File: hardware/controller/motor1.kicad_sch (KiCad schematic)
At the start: 55 parts, among them J5 Conn_01x01, J6 Conn_01x01, J7 Conn_01x01, J8 Conn_01x09, Q2 IPD90N04S4L04, Q3 IPD90N04S4L04, Q4 IPD90N04S4L04, Q5 IPD90N04S4L04, Q6 IPD90N04S4L04, Q7 IPD90N04S4L04, U10 MCP6541, U11 LM2105D, U12 MCP6541, U13 LM2105D, U8 MCP6541, U9 LM2105D

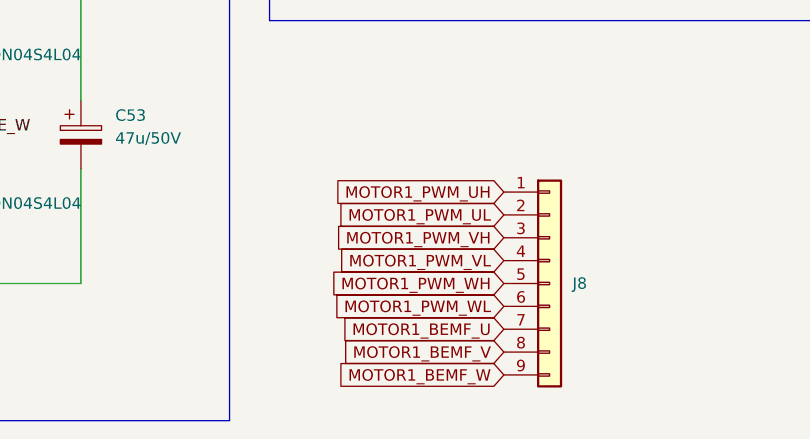
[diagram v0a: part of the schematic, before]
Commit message: wip routing power stages
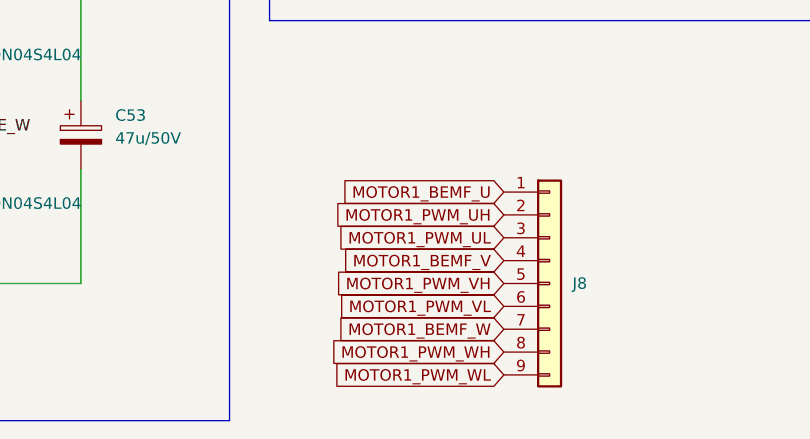
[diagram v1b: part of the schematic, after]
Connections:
- net MOTOR1_BEMF_U: now also J8.1 (Pin_1); no longer J8.7 (Pin_7)
- net MOTOR1_BEMF_V: now also J8.4 (Pin_4); no longer J8.8 (Pin_8)
- net MOTOR1_BEMF_W: now also J8.7 (Pin_7); no longer J8.9 (Pin_9)
- net MOTOR1_PWM_UH: now also J8.2 (Pin_2); no longer J8.1 (Pin_1)
- net MOTOR1_PWM_UL: now also J8.3 (Pin_3); no longer J8.2 (Pin_2)
- net MOTOR1_PWM_VH: now also J8.5 (Pin_5); no longer J8.3 (Pin_3)
- net MOTOR1_PWM_VL: now also J8.6 (Pin_6); no longer J8.4 (Pin_4)
- net MOTOR1_PWM_WH: now also J8.8 (Pin_8); no longer J8.5 (Pin_5)
- net MOTOR1_PWM_WL: now also J8.9 (Pin_9); no longer J8.6 (Pin_6)
